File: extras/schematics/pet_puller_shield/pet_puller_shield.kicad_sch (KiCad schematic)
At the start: 16 parts, among them J1 Jack-DC, J2 Conn_01x02, J3 Conn_01x02, J4 Conn_01x02, J5 Conn_01x04, Q1 IRF540N, U1 LM317_TO-220, U2 MX1508_module

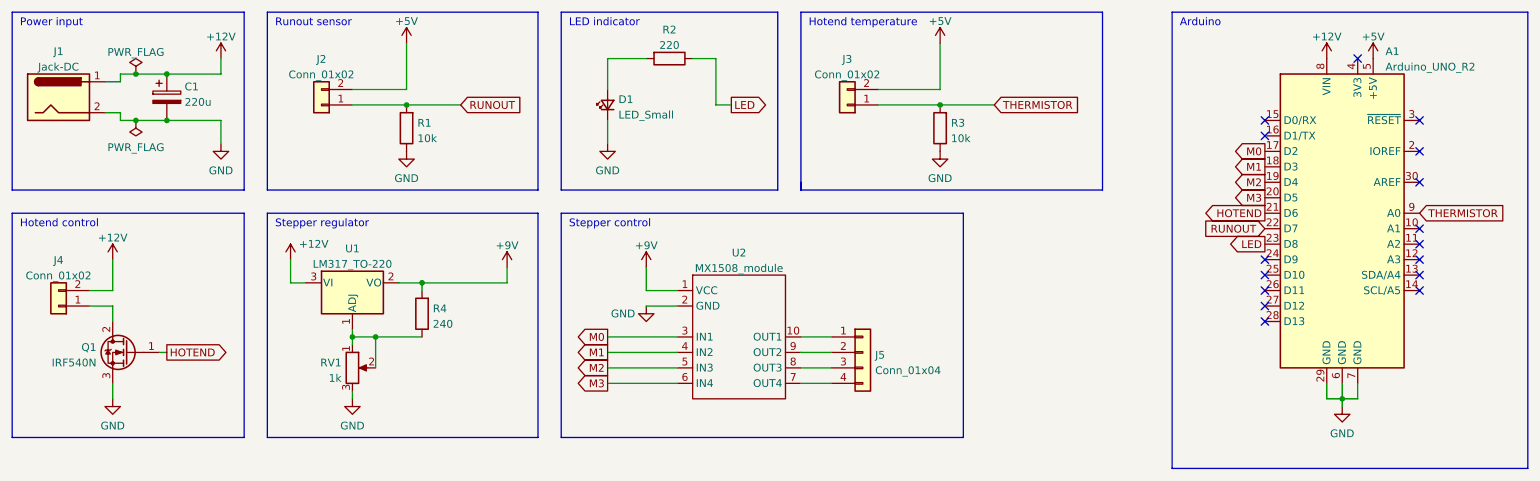
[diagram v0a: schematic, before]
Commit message: Updated schematics
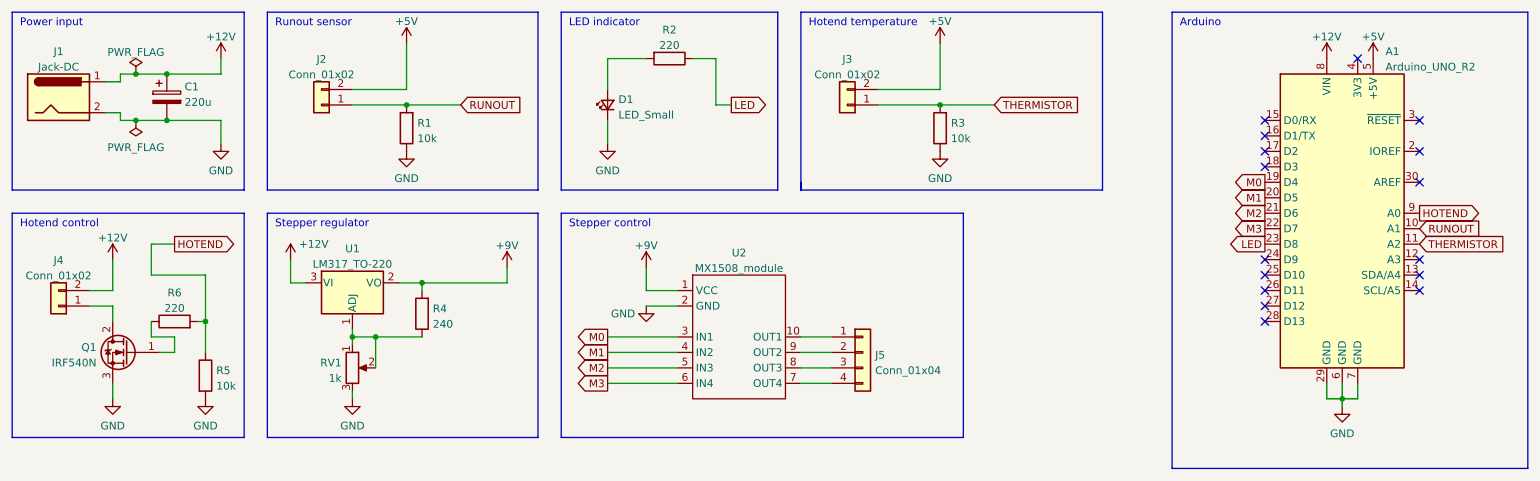
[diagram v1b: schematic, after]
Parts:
- added R5: 10k, Resistor_THT:R_Axial_DIN0204_L3.6mm_D1.6mm_P5.08mm_Horizontal, symbol Device:R
- added R6: 220, Resistor_THT:R_Axial_DIN0204_L3.6mm_D1.6mm_P5.08mm_Horizontal, symbol Device:R
- Q1, U1: footprint Package_TO_SOT_THT:TO-220-3_Vertical -> Package_TO_SOT_THT:TO-220-3_Horizontal_TabDown
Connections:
- net GND: now also R5.2
- net HOTEND: now also A1.9 (A0), R5.1, R6.2; no longer A1.21 (D6), Q1.1 (G)
- net M0: now also A1.19 (D4); no longer A1.17 (D2)
- net M1: now also A1.20 (D5); no longer A1.18 (D3)
- net M2: now also A1.21 (D6); no longer A1.19 (D4)
- net M3: now also A1.22 (D7); no longer A1.20 (D5)
- net RUNOUT: now also A1.10 (A1); no longer A1.22 (D7)
- net THERMISTOR: now also A1.11 (A2); no longer A1.9 (A0)
- new net: Q1.1 (G), R6.1
